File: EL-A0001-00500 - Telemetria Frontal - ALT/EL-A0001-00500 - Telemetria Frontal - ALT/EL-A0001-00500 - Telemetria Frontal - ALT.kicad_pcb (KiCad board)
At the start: 2 copper layers, 100 x 100 mm, 29 parts, among them J1 1-776087-1, J2 UART, U1 YAAJ_BluePill, U2 MP1584, U3 TJA1050-Module, U4 LM324, U5 LM324

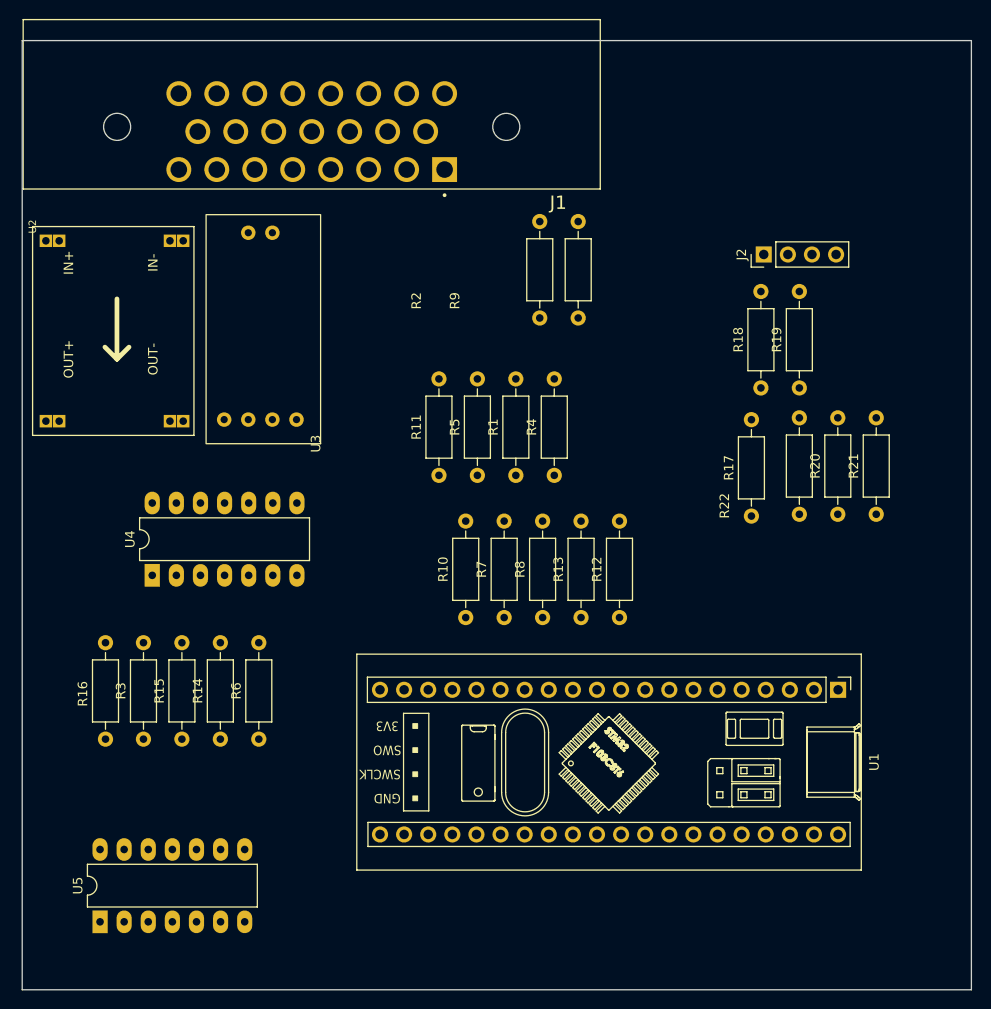
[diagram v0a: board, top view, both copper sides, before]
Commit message: MOD: placa de telemetria frontal ALT
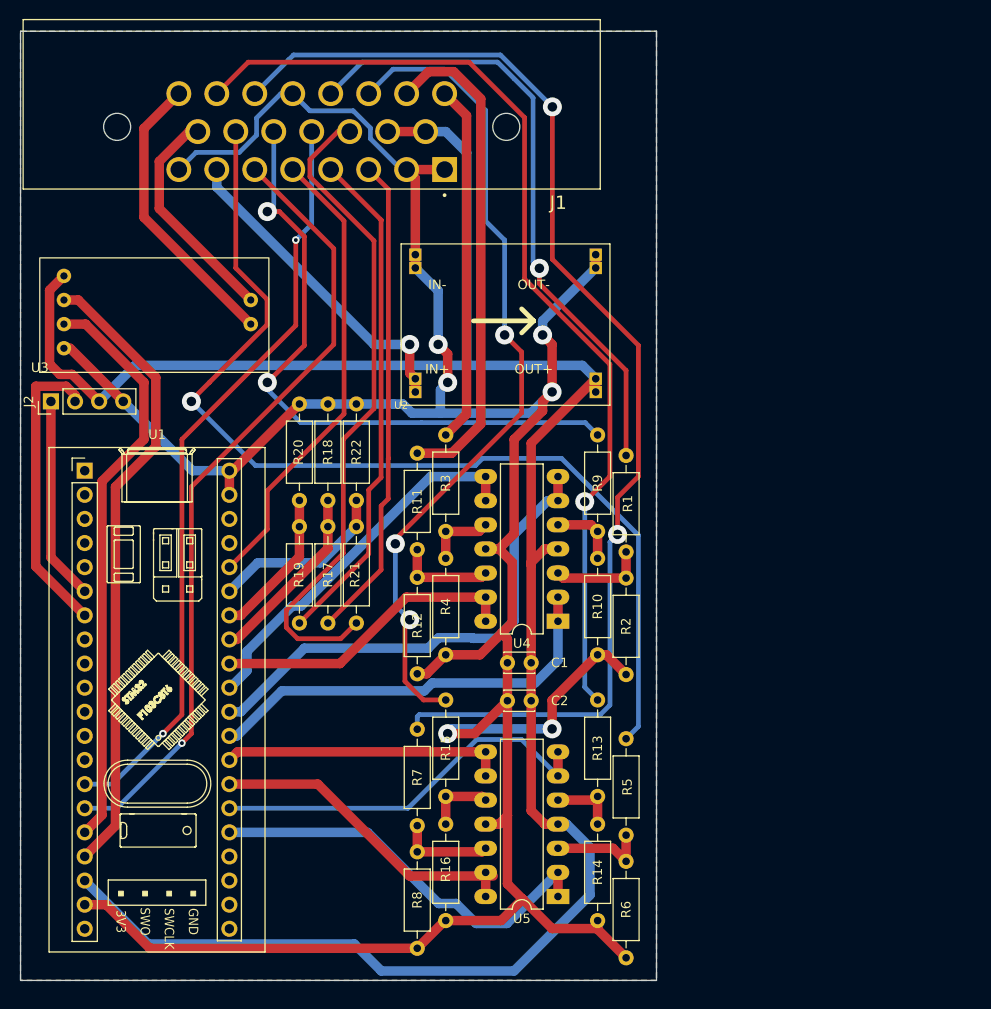
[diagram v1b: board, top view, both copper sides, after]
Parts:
- added C1: 100nF, Capacitor_THT:C_Disc_D3.0mm_W2.0mm_P2.50mm, F.Cu at (88.8, 118.5)
- added C2: 100nF, Capacitor_THT:C_Disc_D3.0mm_W2.0mm_P2.50mm, F.Cu at (88.8, 122.5)
- moved U1 82.7 mm to (41.8, 98.3), turned to 0 degrees
- moved J2 76.7 mm to (38.2, 91.0)
- moved R19 58.2 mm to (64.4, 114.3)
- moved R20 56.7 mm to (64.4, 101.4)
- moved R21 56.0 mm to (70.4, 114.3)
- moved U5 48.3 mm to (91.6, 143.2), turned to 180 degrees
- moved R18 47.1 mm to (67.4, 101.4)
- moved R22 46.7 mm to (70.4, 101.4)
- moved R17 46.0 mm to (67.4, 114.3)
- moved R3 45.2 mm to (79.8, 94.5), turned to -90 degrees
- moved U2 43.1 mm to (75.1, 91.4), turned to 0 degrees
- moved U4 43.0 mm to (91.6, 114.2), turned to 180 degrees
- moved R6 40.8 mm to (98.8, 139.5), turned to -90 degrees
- moved R14 40.7 mm to (95.8, 135.5), turned to -90 degrees
- moved R16 36.9 mm to (79.8, 135.5), turned to -90 degrees
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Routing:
- net GND: track 0.00 -> 314.4 mm, vias 0 -> 6
- net +5V: track 0.00 -> 229.7 mm
- net ADC_IN_3: track 0.00 -> 126.2 mm, vias 0 -> 2
- net ADC_IN_1: track 0.00 -> 108.6 mm, vias 0 -> 1
- net ADC_IN_2: track 0.00 -> 103.0 mm, vias 0 -> 1
- net TPS_IN_1: track 0.00 -> 88.4 mm, vias 0 -> 3
- net PWT_IN_2: track 0.00 -> 83.6 mm, vias 0 -> 1
- net PWT_IN_4: track 0.00 -> 80.4 mm, vias 0 -> 2
- net SHUT_IN: track 0.00 -> 69.9 mm
- net FREIOS_IN_1: track 0.00 -> 68.2 mm, vias 0 -> 2
- net CAN_TX: track 0.00 -> 66.6 mm
- net TPS_IN_2: track 0.00 -> 66.0 mm, vias 0 -> 1
- net CAN_RX: track 0.00 -> 61.0 mm
- net INERTIA_IN: track 0.00 -> 53.6 mm
- net FREIOS_IN_3: track 0.00 -> 52.2 mm
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- added copper zone on B.Cu, net GND
- added copper zone on F.Cu, net GND
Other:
- board size 100 x 100 mm -> 67 x 100 mm

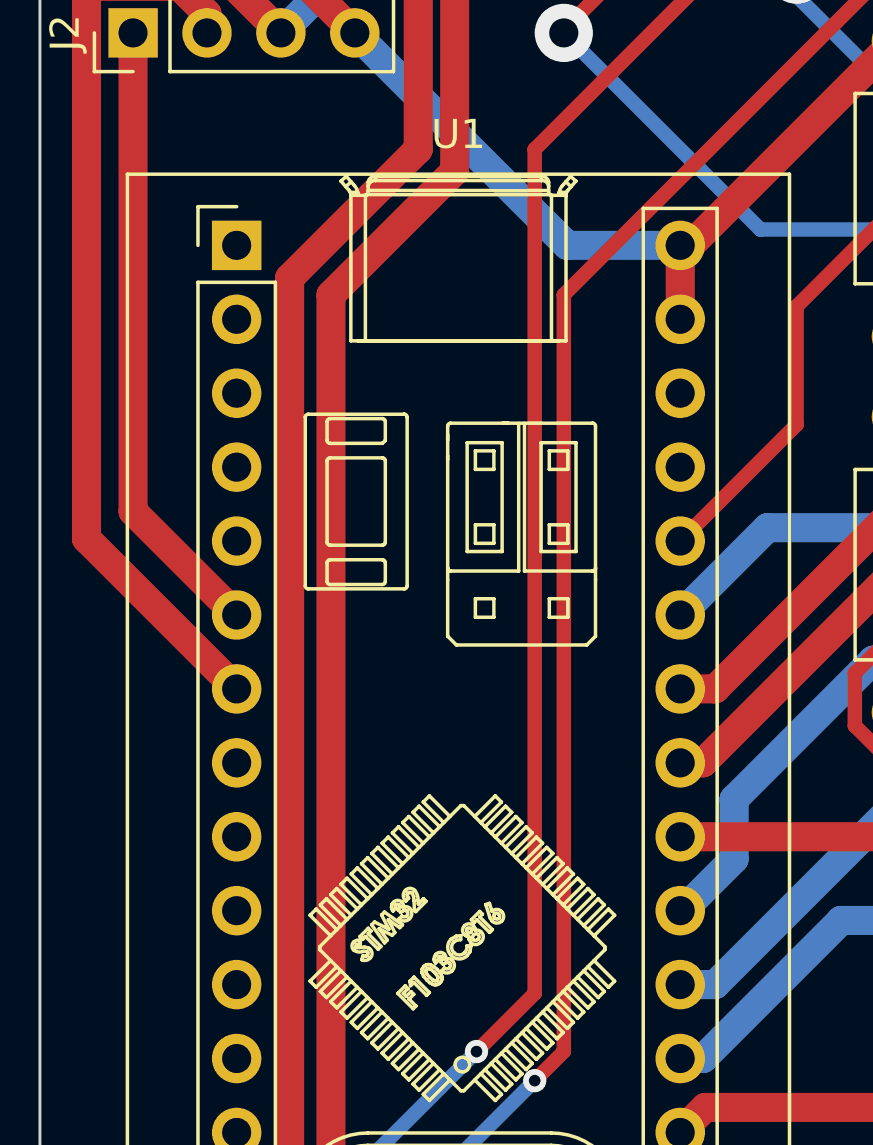
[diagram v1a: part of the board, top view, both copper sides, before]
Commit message: AA
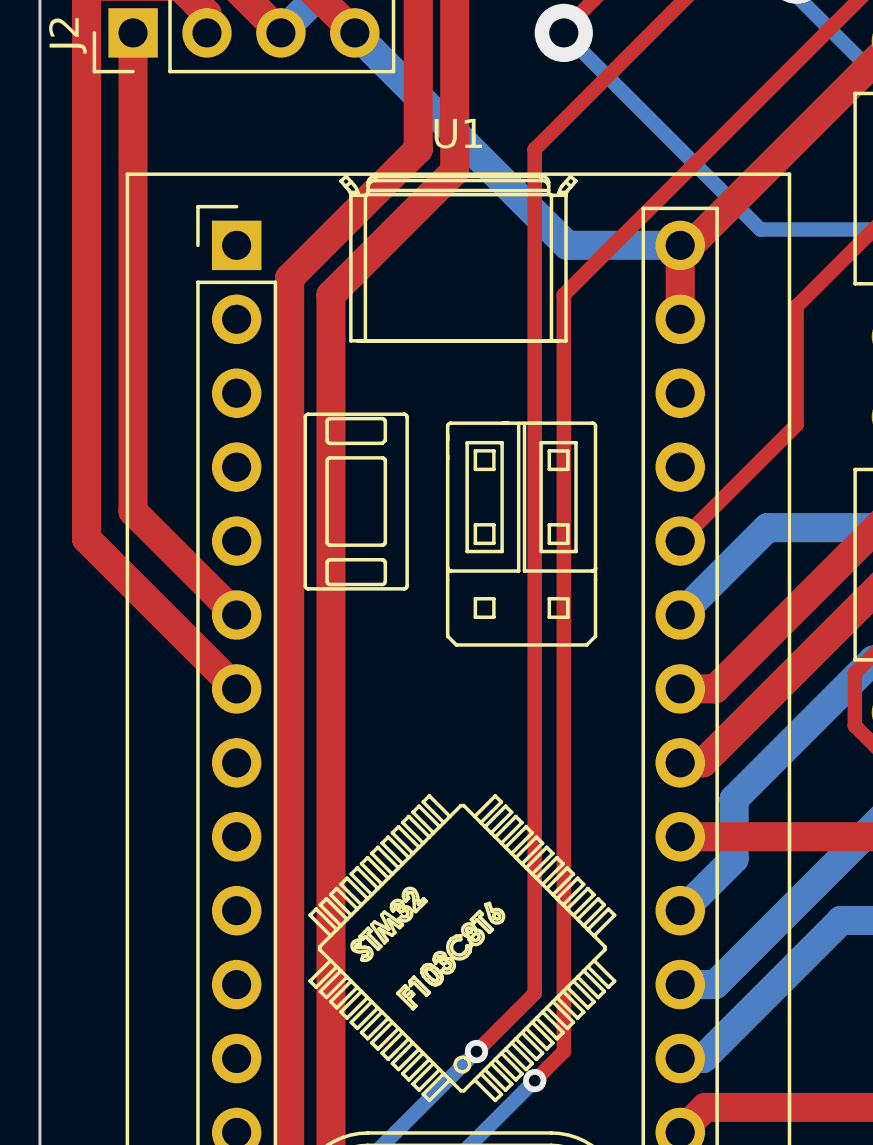
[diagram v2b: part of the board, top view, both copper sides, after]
